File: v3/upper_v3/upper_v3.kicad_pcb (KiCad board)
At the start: 2 copper layers, 35.6 x 68.6 mm, 3 parts, among them J1 Conn_01x18, J2 Conn_01x09_Male, J3 Conn_01x09_Male

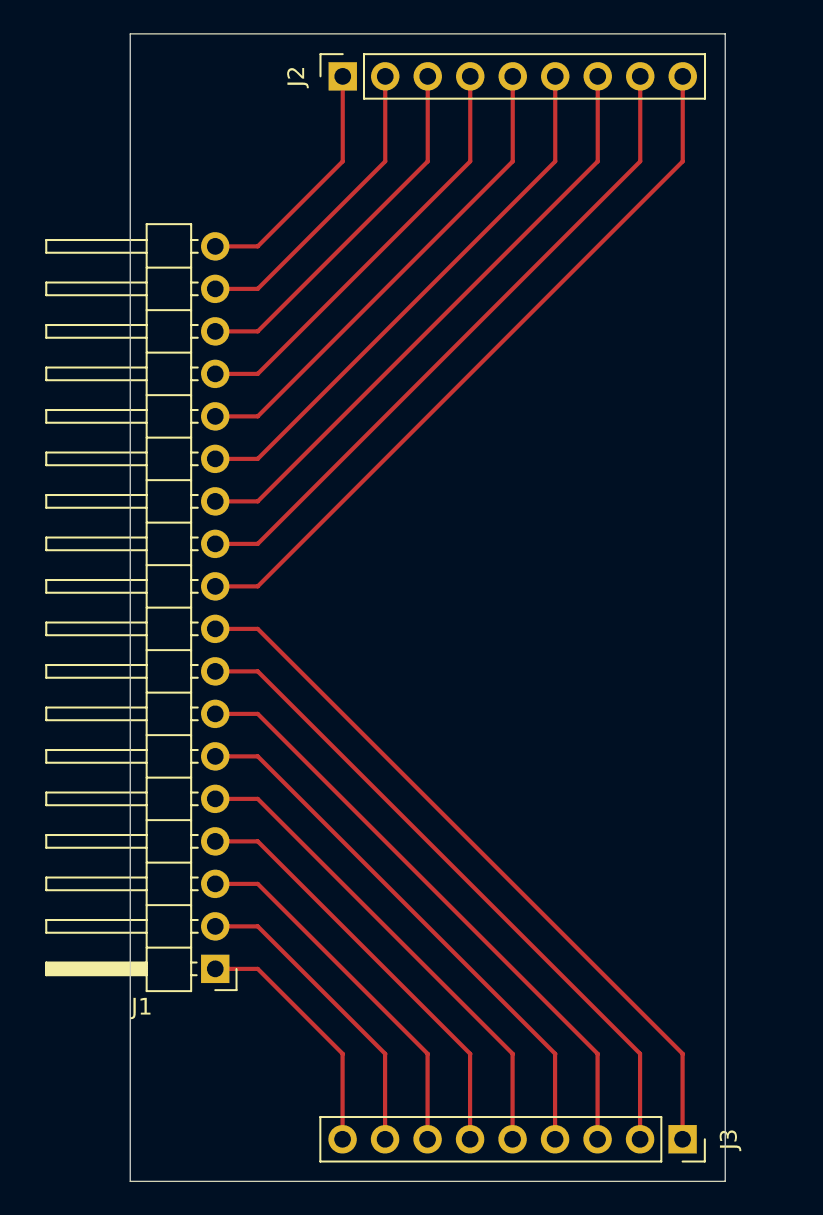
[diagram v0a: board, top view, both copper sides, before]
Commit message: Complete Toast PCB
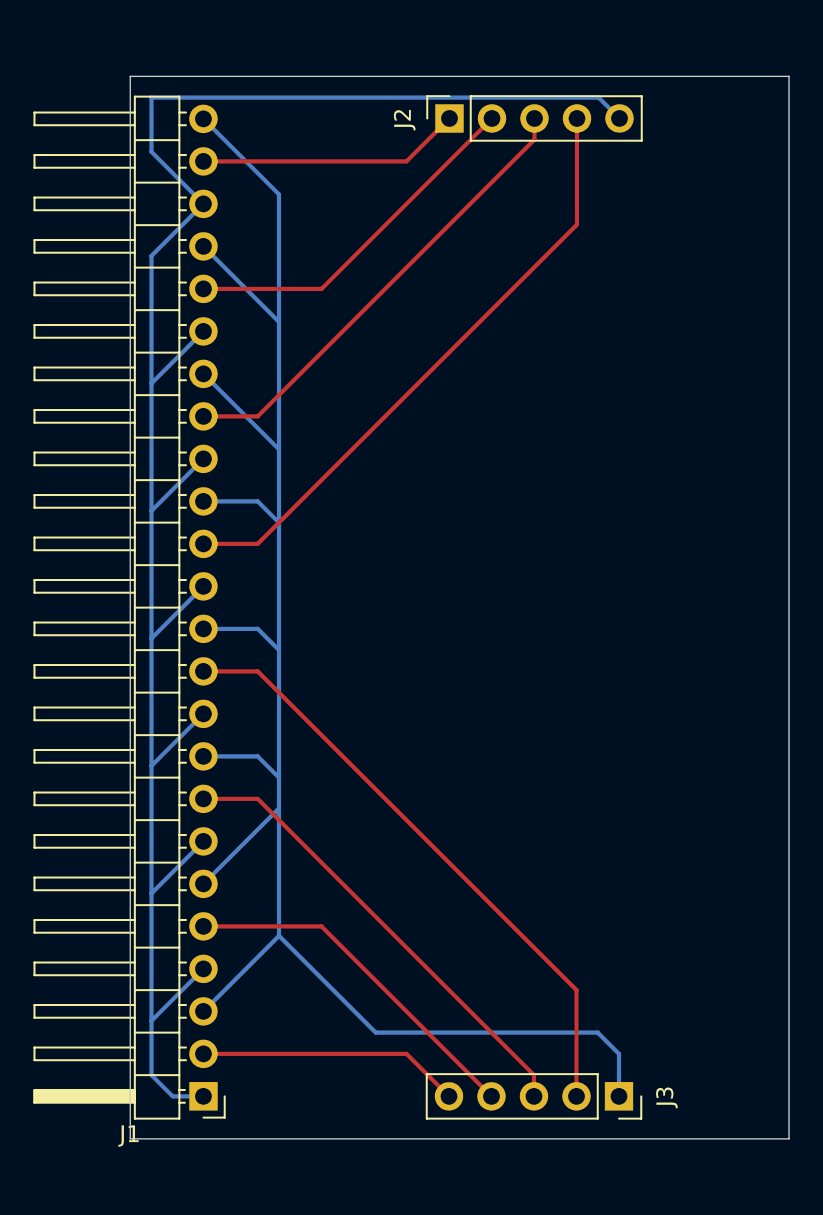
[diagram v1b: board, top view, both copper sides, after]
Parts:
- J1: value Conn_01x18 -> Conn_01x24; footprint Connector_PinHeader_2.54mm:PinHeader_1x18_P2.54mm_Horizontal -> Connector_PinHeader_2.54mm:PinHeader_1x24_P2.54mm_Horizontal
- J2, J3: value Conn_01x09_Male -> Conn_01x05_Female; footprint Connector_PinSocket_2.54mm:PinSocket_1x09_P2.54mm_Vertical -> Connector_PinSocket_2.54mm:PinSocket_1x05_P2.54mm_Vertical
- moved J1 7.65 mm to (121.2, 127.0)
- moved J2 6.86 mm to (135.9, 68.6)
- moved J3 4.58 mm to (146.1, 127.0)
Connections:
- J1 pad 10: Net-(J1-Pad10) -> Net-(J1-Pad1)
- J1 pad 13: Net-(J1-Pad13) -> Net-(J1-Pad1)
- J1 pad 15: Net-(J1-Pad15) -> Net-(J1-Pad12)
- J1 pad 16: Net-(J1-Pad16) -> Net-(J1-Pad1)
- J1 pad 18: Net-(J1-Pad18) -> Net-(J1-Pad12)
- J1 pad 3: Net-(J1-Pad3) -> Net-(J1-Pad12)
- J1 pad 4: Net-(J1-Pad4) -> Net-(J1-Pad1)
- J1 pad 6: Net-(J1-Pad6) -> Net-(J1-Pad12)
- J1 pad 7: Net-(J1-Pad7) -> Net-(J1-Pad1)
- J1 pad 9: Net-(J1-Pad9) -> Net-(J1-Pad12)
- J2 pad 1: Net-(J1-Pad18) -> Net-(J1-Pad23)
- J2 pad 2: Net-(J1-Pad17) -> Net-(J1-Pad20)
- J2 pad 3: Net-(J1-Pad16) -> Net-(J1-Pad17)
- J2 pad 4: Net-(J1-Pad15) -> Net-(J1-Pad14)
- J2 pad 5: Net-(J1-Pad14) -> Net-(J1-Pad1)
- J3 pad 1: Net-(J1-Pad9) -> Net-(J1-Pad12)
- J3 pad 2: Net-(J1-Pad8) -> Net-(J1-Pad11)
- J3 pad 3: Net-(J1-Pad7) -> Net-(J1-Pad8)
- J3 pad 4: Net-(J1-Pad6) -> Net-(J1-Pad5)
- J3 pad 5: Net-(J1-Pad5) -> Net-(J1-Pad2)
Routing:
- net Net-(J1-Pad1): track 14.8 -> 119.5 mm
- net Net-(J1-Pad12): track 36.4 -> 117.1 mm
- net Net-(J1-Pad9): track 43.6 -> 0.00 mm
- net Net-(J1-Pad10): track 43.5 -> 0.00 mm
- net Net-(J1-Pad7): track 36.4 -> 0.00 mm
- net Net-(J1-Pad6): track 32.8 -> 0.00 mm
- net Net-(J1-Pad13): track 32.8 -> 0.00 mm
- net Net-(J1-Pad4): track 25.6 -> 0.00 mm
- net Net-(J1-Pad15): track 25.6 -> 0.00 mm
- net Net-(J1-Pad3): track 22.0 -> 0.00 mm
- net Net-(J1-Pad16): track 22.0 -> 0.00 mm
- net Net-(J1-Pad20): track 0.00 -> 21.5 mm
- net Net-(J1-Pad23): track 0.00 -> 15.8 mm
- net Net-(J1-Pad18): track 14.8 -> 0.00 mm
- net Net-(J1-Pad8): track 40.0 -> 27.9 mm
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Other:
- board size 35.6 x 68.6 mm -> 39.4 x 63.5 mm
